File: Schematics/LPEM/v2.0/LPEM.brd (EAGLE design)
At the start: 55.9 x 100.6 mm, 33 parts, among them IC3 PCA9600SO8

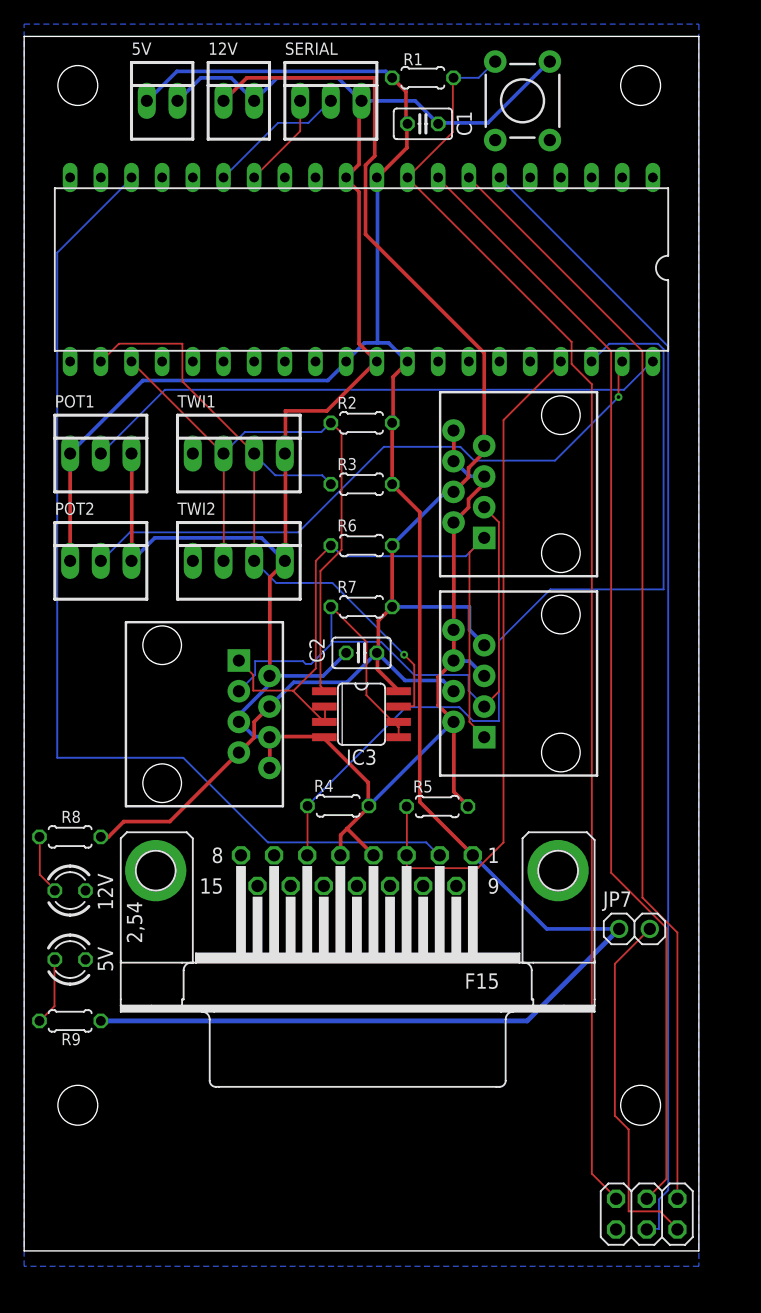
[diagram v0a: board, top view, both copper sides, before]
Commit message: final LPEM
git-svn-id: https://svn.circlemud.org/svn/rocket/trunk@835 46170a15-b891-4bf7-af97-fd374ce181e0
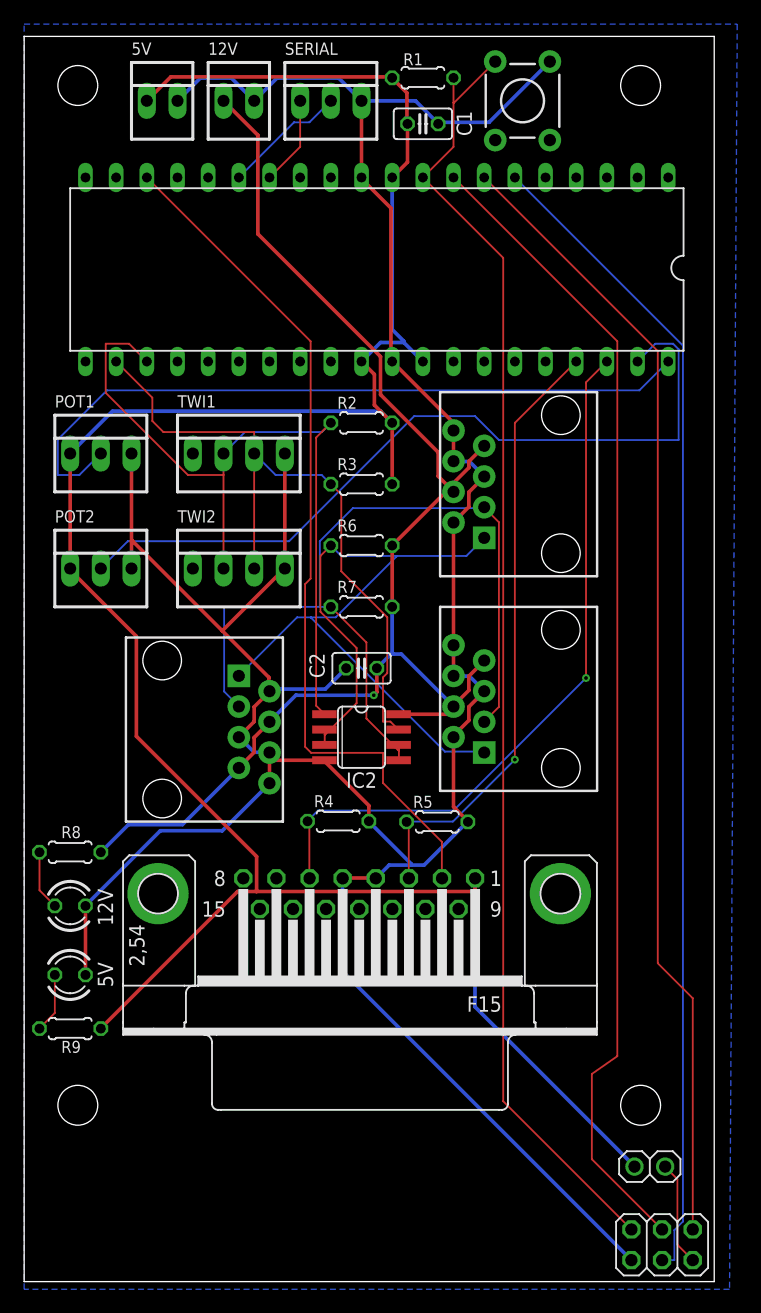
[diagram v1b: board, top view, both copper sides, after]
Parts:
- removed IC3: PCA9600SO8, 4534_I2C2:SO08
- added IC2: PCA9600SO8, 4534_I2C2:SO08
- moved JP7 19.7 mm to (51.8, -0.64)
- moved JP10 2.84 mm to (52.8, -7.11)
- moved X1 1.91 mm to (27.7, 22.0)
- moved 12V1 1.27 mm to (3.81, 21.0)
- moved R8 1.27 mm to (3.81, 25.4)
- moved 5V1 1.27 mm to (3.81, 15.2)
- moved IC1 1.27 mm to (29.2, 73.7)
- moved R4 1.27 mm to (26.0, 28.0)
- moved R5 1.27 mm to (34.2, 27.9)
- moved C2 1.27 mm to (27.9, 40.6)
- moved U$1 1.27 mm to (44.5, 38.1)
- moved U$3 1.27 mm to (11.4, 35.6)
- moved R9 0.63 mm to (3.81, 10.8)
- moved POT2 0.63 mm to (6.35, 48.9)
- moved TWI2 0.63 mm to (17.8, 48.9)
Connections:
- net +12V: now also IC2.8; no longer IC3.8
- net GND: now also IC2.4; no longer IC3.4
- net SCL: now also IC2.7; no longer IC3.7
- net SCL_12V: now also IC2.5, IC2.6; no longer IC3.5, IC3.6
- net SDA: now also IC2.1; no longer IC3.1
- net SDA_12V: now also IC2.2, IC2.3; no longer IC3.2, IC3.3
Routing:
- net GND: track 202.6 -> 263.1 mm
- net N$4: track 29.8 -> 8.69 mm
- net SDA_12V: track 55.9 -> 69.6 mm
- net JOYTRIG: track 85.6 -> 72.0 mm
- net N$2: track 52.5 -> 65.6 mm, vias 1 -> 0
- net N$6: track 72.5 -> 59.7 mm, vias 0 -> 1
- net SCL_12V: track 60.0 -> 72.2 mm
- net SDA: track 53.2 -> 65.1 mm
- net N$1: track 48.9 -> 60.5 mm
- net +12V: track 121.0 -> 111.1 mm, vias 0 -> 1
- net VCC: track 191.4 -> 199.5 mm
- net N$3: track 55.9 -> 50.9 mm, vias 0 -> 1
- net SCK: track 93.1 -> 96.2 mm
- net RESET: track 105.7 -> 108.4 mm
- net MISO: track 91.7 -> 94.3 mm
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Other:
- board size 55.9 x 100.6 mm -> 57.1 x 103.1 mm
